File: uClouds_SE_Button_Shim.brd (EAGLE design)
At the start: 40 x 110.5 mm, 0 parts

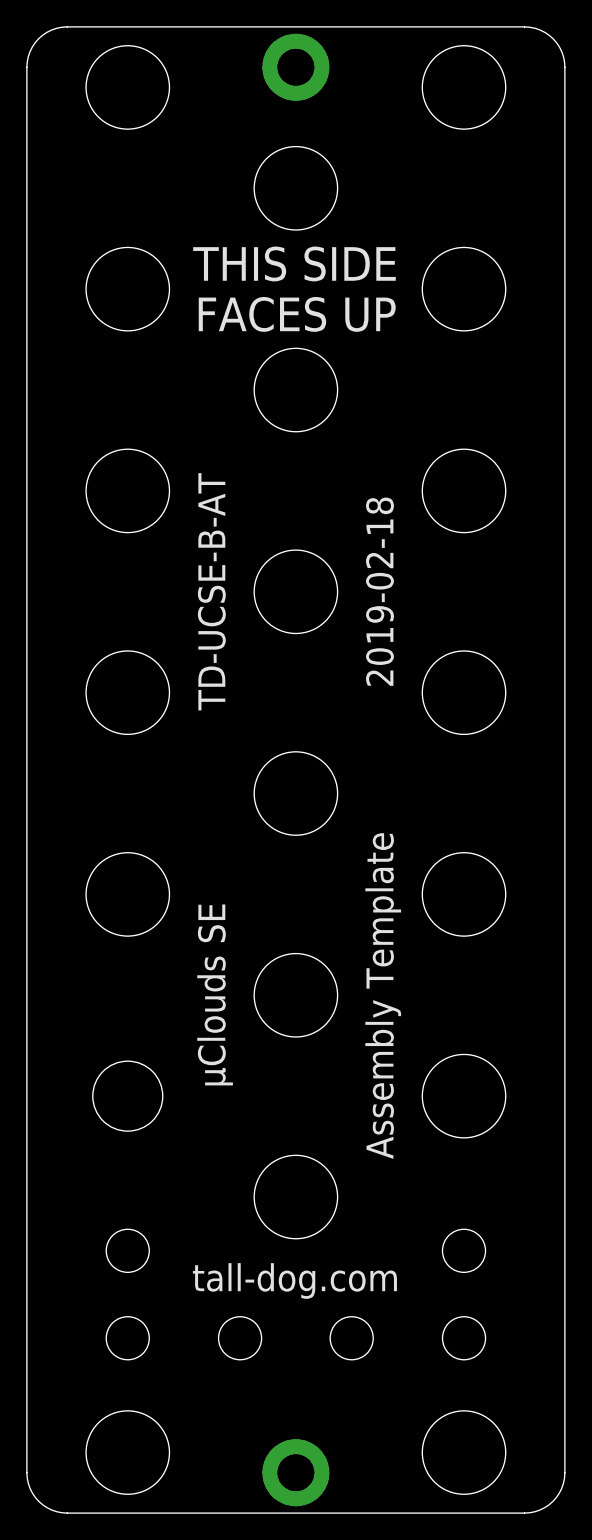
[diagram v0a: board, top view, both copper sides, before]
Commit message: assembly process updates
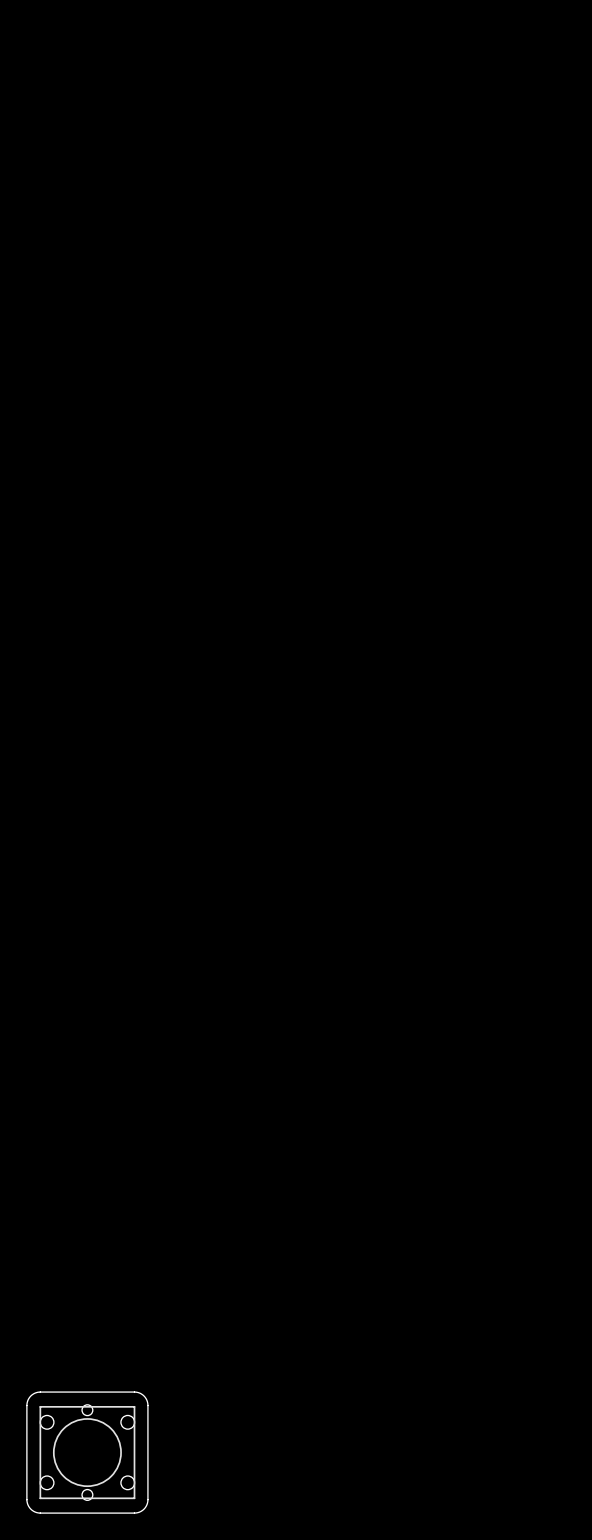
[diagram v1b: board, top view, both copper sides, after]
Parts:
- added E$1: (no value), uClouds_SE_Library:TL1265-HOLES
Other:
- board size 40 x 110.5 mm -> 9 x 9 mm
- board text removed: "2019-02-18"
- board text removed: "Assembly Template"
- board text removed: "TD-UCSE-B-AT"
- board text removed: "THIS SIDE FACES DOWN"
- board text removed: "THIS SIDE FACES UP"
- board text removed: "tall-dog.com"
- board text removed: "µClouds SE"
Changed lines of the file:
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@@
 <?xml version="1.0" encoding="utf-8"?>
 <!DOCTYPE eagle SYSTEM "eagle.dtd">
-<eagle version="9.3.1">
+<eagle version="9.2.2">
 <drawing>
 <settings>
@@
 <setting verticaltext="up"/>
 </settings>
-<grid distance="0.5" unitdist="mm" unit="mm" style="lines" multiple="1" display="yes" altdistance="0.025" altunitdist="inch" altunit="inch"/>
+<grid distance="0.5" unitdist="mm" unit="mm" style="lines" multiple="1" display="yes" altdistance="5" altunitdist="mil" altunit="mil"/>
 <layers>
 <layer number="1" name="Top" color="4" fill="1" visible="yes" active="yes"/>
-<layer number="2" name="Route2" color="1" fill="3" visible="no" active="no"/>
-<layer number="15" name="Route15" color="4" fill="6" visible="no" active="no"/>
 <layer number="16" name="Bottom" color="1" fill="1" visible="yes" active="yes"/>
 <layer number="17" name="Pads" color="2" fill="1" visible="yes" active="yes"/>
 <layer number="18" name="Vias" color="2" fill="1" visible="yes" active="yes"/>
 <layer number="19" name="Unrouted" color="6" fill="1" visible="yes" active="yes"/>
-<layer number="20" name="Dimension" color="15" fill="1" visible="yes" active="yes"/>
+<layer number="20" name="Dimension" color="24" fill="1" visible="yes" active="yes"/>
 <layer number="21" name="tPlace" color="7" fill="1" visible="yes" active="yes"/>
-<layer number="22" name="bPlace" color="6" fill="1" visible="yes" active="yes"/>
+<layer number="22" name="bPlace" color="7" fill="1" visible="yes" active="yes"/>
 <layer number="23" name="tOrigins" color="15" fill="1" visible="yes" active="yes"/>
 <layer number="24" name="bOrigins" color="15" fill="1" visible="yes" active="yes"/>
@@
 <layer number="47" name="Measures" color="7" fill="1" visible="yes" active="yes"/>
 <layer number="48" name="Document" color="7" fill="1" visible="yes" active="yes"/>
-<layer number="49" name="Reference" color="5" fill="1" visible="yes" active="yes"/>
+<layer number="49" name="Reference" color="7" fill="1" visible="yes" active="yes"/>
 <layer number="51" name="tDocu" color="7" fill="1" visible="yes" active="yes"/>
 <layer number="52" name="bDocu" color="7" fill="1" visible="yes" active="yes"/>
@@
 <board>
 <plain>
-<wire x1="37" y1="110.5" x2="3" y2="110.5" width="0" layer="20"/>
-<wire x1="0" y1="107.5" x2="0" y2="3" width="0" layer="20"/>
-<wire x1="40" y1="107.5" x2="40" y2="3" width="0" layer="20"/>
-<wire x1="37" y1="0" x2="3" y2="0" width="0" layer="20"/>
-<wire x1="3" y1="0" x2="0" y2="3" width="0" layer="20" curve="-90"/>
-<wire x1="40" y1="3" x2="37" y2="0" width="0" layer="20" curve="-90"/>
-<wire x1="37" y1="110.5" x2="40" y2="107.5" width="0" layer="20" curve="-90"/>
-<wire x1="0" y1="107.5" x2="3" y2="110.5" width="0" layer="20" curve="-90"/>
-<hole x="7.5" y="106" drill="6.2"/>
-<hole x="7.5" y="91" drill="6.2"/>
-<hole x="7.5" y="76" drill="6.2"/>
-<hole x="7.5" y="61" drill="6.2"/>
-<hole x="7.5" y="46" drill="6.2"/>
-<hole x="20" y="98.5" drill="6.2"/>
-<hole x="32.5" y="106" drill="6.2"/>
-<hole x="32.5" y="91" drill="6.2"/>
-<hole x="20" y="83.5" drill="6.2"/>
-<hole x="32.5" y="76" drill="6.2"/>
-<hole x="20" y="68.5" drill="6.2"/>
-<hole x="32.5" y="61" drill="6.2"/>
-<hole x="20" y="53.5" drill="6.2"/>
-<hole x="32.5" y="46" drill="6.2"/>
-<hole x="20" y="38.5" drill="6.2"/>
-<hole x="7.5" y="13" drill="3.2"/>
-<text x="13.75" y="38.5" size="2" layer="21" rot="R90" align="center">µClouds SE</text>
-<text x="20" y="17.5" size="2" layer="21" align="center">tall-dog.com</text>
-<hole x="32.5" y="31" drill="6.2"/>
-<hole x="20" y="23.5" drill="6.2"/>
-<hole x="32.5" y="13" drill="3.2"/>
-<hole x="15.85" y="13" drill="3.2"/>
-<hole x="24.15" y="13" drill="3.2"/>
-<hole x="7.5" y="4.5" drill="6.2"/>
-<hole x="32.5" y="4.5" drill="6.2"/>
-<hole x="7.5" y="19.5" drill="3.2"/>
-<hole x="32.5" y="19.5" drill="3.2"/>
-<hole x="7.5" y="31" drill="5.2"/>
-<text x="26.25" y="38.5" size="2" layer="21" rot="R90" align="center">Assembly Template</text>
-<text x="13.75" y="68.5" size="2" layer="21" rot="R90" align="center">TD-UCSE-B-AT</text>
-<text x="26.25" y="68.5" size="2" layer="21" rot="R90" align="center">2019-02-18</text>
-<text x="20" y="91" size="2.5" layer="21" ratio="10" rot="R180" align="center">THIS SIDE
-FACES UP</text>
-<text x="20" y="91" size="2" layer="22" ratio="10" rot="MR180" align="center">THIS SIDE
-FACES DOWN</text>
-<text x="26.25" y="68.5" size="2" layer="22" rot="MR90" align="center">TD-UCSE-B-AT</text>
-<text x="13.75" y="68.5" size="2" layer="22" rot="MR90" align="center">2019-02-18</text>
-<text x="26.25" y="38.5" size="2" layer="22" rot="MR90" align="center">µClouds SE</text>
-<text x="13.75" y="38.5" size="2" layer="22" rot="MR90" align="center">Assembly Template</text>
-<text x="20" y="17.5" size="2" layer="22" rot="MR0" align="center">tall-dog.com</text>
+<wire x1="0" y1="1" x2="0" y2="8" width="0" layer="20"/>
+<wire x1="1" y1="9" x2="8" y2="9" width="0" layer="20"/>
+<wire x1="9" y1="8" x2="9" y2="1" width="0" layer="20"/>
+<wire x1="8" y1="0" x2="1" y2="0" width="0" layer="20"/>
+<wire x1="0" y1="8" x2="1" y2="9" width="0" layer="20" curve="-90"/>
+<wire x1="1" y1="0" x2="0" y2="1" width="0" layer="20" curve="-90"/>
+<wire x1="9" y1="1" x2="8" y2="0" width="0" layer="20" curve="-90"/>
+<wire x1="8" y1="9" x2="9" y2="8" width="0" layer="20" curve="-90"/>
 </plain>
 <attributes>
@@
 </class>
 </classes>
-<designrules name="default *">
+<designrules name="default">
 <description language="de">&lt;b&gt;EAGLE Design Rules&lt;/b&gt;
 &lt;p&gt;
@@
 <param name="mtCopper" value="0.035mm 0.035mm 0.035mm 0.035mm 0.035mm 0.035mm 0.035mm 0.035mm 0.035mm 0.035mm 0.035mm 0.035mm 0.035mm 0.035mm 0.035mm 0.035mm"/>
 <param name="mtIsolate" value="1.5mm 0.15mm 0.2mm 0.15mm 0.2mm 0.15mm 0.2mm 0.15mm 0.2mm 0.15mm 0.2mm 0.15mm 0.2mm 0.15mm 0.2mm"/>
-<param name="mdWireWire" value="8mil"/>
-<param name="mdWirePad" value="8mil"/>
-<param name="mdWireVia" value="8mil"/>
-<param name="mdPadPad" value="8mil"/>
-<param name="mdPadVia" value="8mil"/>
-<param name="mdViaVia" value="8mil"/>
-<param name="mdSmdPad" value="8mil"/>
-<param name="mdSmdVia" value="8mil"/>
-<param name="mdSmdSmd" value="8mil"/>
-<param name="mdViaViaSameLayer" value="8mil"/>
+<param name="mdWireWire" value="6mil"/>
+<param name="mdWirePad" value="6mil"/>
+<param name="mdWireVia" value="6mil"/>
+<param name="mdPadPad" value="6mil"/>
+<param name="mdPadVia" value="6mil"/>
+<param name="mdViaVia" value="6mil"/>
+<param name="mdSmdPad" value="6mil"/>
+<param name="mdSmdVia" value="6mil"/>
+<param name="mdSmdSmd" value="6mil"/>
+<param name="mdViaViaSameLayer" value="6mil"/>
 <param name="mnLayersViaInSmd" value="2"/>
-<param name="mdCopperDimension" value="0.25mm"/>
-<param name="mdDrill" value="8mil"/>
+<param name="mdCopperDimension" value="40mil"/>
+<param name="mdDrill" value="6mil"/>
 <param name="mdSmdStop" value="0mil"/>
-<param name="msWidth" value="10mil"/>
-<param name="msDrill" value="0.3mm"/>
+<param name="msWidth" value="6mil"/>
+<param name="msDrill" value="0.35mm"/>
 <param name="msMicroVia" value="9.99mm"/>
 <param name="msBlindViaRatio" value="0.5"/>
@@
 <param name="rvMicroViaOuter" value="0.25"/>
 <param name="rvMicroViaInner" value="0.25"/>
-<param name="rlMinPadTop" value="6mil"/>
+<param name="rlMinPadTop" value="10mil"/>
 <param name="rlMaxPadTop" value="20mil"/>
-<param name="rlMinPadInner" value="6mil"/>
+<param name="rlMinPadInner" value="10mil"/>
 <param name="rlMaxPadInner" value="20mil"/>
-<param name="rlMinPadBottom" value="6mil"/>
+<param name="rlMinPadBottom" value="10mil"/>
 <param name="rlMaxPadBottom" value="20mil"/>
-<param name="rlMinViaOuter" value="6mil"/>
+<param name="rlMinViaOuter" value="8mil"/>
 <param name="rlMaxViaOuter" value="20mil"/>
-<param name="rlMinViaInner" value="6mil"/>
+<param name="rlMinViaInner" value="8mil"/>
 <param name="rlMaxViaInner" value="20mil"/>
 <param name="rlMinMicroViaOuter" value="4mil"/>
@@
 <param name="psElongationLong" value="100"/>
 <param name="psElongationOffset" value="100"/>
-<param name="mvStopFrame" value="0"/>
+<param name="mvStopFrame" value="1"/>
 <param name="mvCreamFrame" value="0"/>
-<param name="mlMinStopFrame" value="0mil"/>
-<param name="mlMaxStopFrame" value="0mil"/>
+<param name="mlMinStopFrame" value="4mil"/>
+<param name="mlMaxStopFrame" value="4mil"/>
 <param name="mlMinCreamFrame" value="0mil"/>
 <param name="mlMaxCreamFrame" value="0mil"/>
@@
 </autorouter>
 <elements>
+<element name="E$1" library="uClouds_SE_Library" package="TL1265-HOLES" value="" x="4.5" y="4.5" smashed="yes"/>
 </elements>
 <signals>
-<signal name="S$1">
-<via x="20" y="107.5" extent="1-16" drill="2.75" diameter="5"/>
-</signal>
-<signal name="S$2">
-<via x="20" y="3" extent="1-16" drill="2.75" diameter="5"/>
-</signal>
 </signals>
 <mfgpreviewcolors>
@@
 </board>
 </drawing>
-<compatibility>
-<note version="6.3" minversion="6.2.2" severity="warning">
-Since Version 6.2.2 text objects can contain more than one line,
-which will not be processed correctly with this version.
-</note>
-</compatibility>
 </eagle>

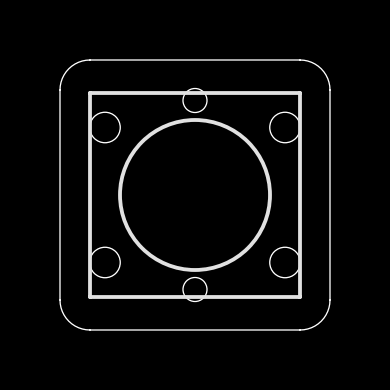
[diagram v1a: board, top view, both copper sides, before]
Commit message: Updates for Revision D
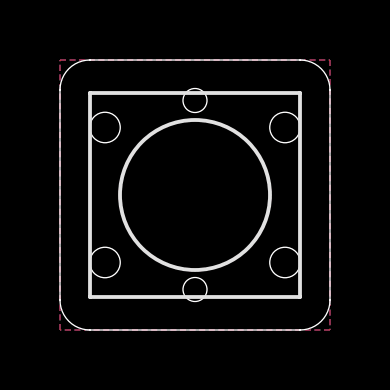
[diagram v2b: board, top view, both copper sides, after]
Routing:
- added copper zone on layer 1, net GND
- added copper zone on layer 16, net GND
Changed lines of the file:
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@@
 <?xml version="1.0" encoding="utf-8"?>
 <!DOCTYPE eagle SYSTEM "eagle.dtd">
-<eagle version="9.2.2">
+<eagle version="9.5.2">
 <drawing>
 <settings>
@@
 </class>
 </classes>
-<designrules name="default">
+<designrules name="default *">
 <description language="de">&lt;b&gt;EAGLE Design Rules&lt;/b&gt;
 &lt;p&gt;
@@
 <param name="mdViaViaSameLayer" value="6mil"/>
 <param name="mnLayersViaInSmd" value="2"/>
-<param name="mdCopperDimension" value="40mil"/>
+<param name="mdCopperDimension" value="12mil"/>
 <param name="mdDrill" value="6mil"/>
 <param name="mdSmdStop" value="0mil"/>
@@
 </elements>
 <signals>
+<signal name="GND">
+<polygon width="0.2" layer="1" isolate="0.2">
+<vertex x="0" y="9"/>
+<vertex x="9" y="9"/>
+<vertex x="9" y="0"/>
+<vertex x="0" y="0"/>
+</polygon>
+<polygon width="0.2" layer="16" isolate="0.2">
+<vertex x="0" y="9"/>
+<vertex x="9" y="9"/>
+<vertex x="9" y="0"/>
+<vertex x="0" y="0"/>
+</polygon>
+</signal>
 </signals>
 <mfgpreviewcolors>
